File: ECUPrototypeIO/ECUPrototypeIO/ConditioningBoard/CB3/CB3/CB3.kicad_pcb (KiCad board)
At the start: 2 copper layers, 123.2 x 101.6 mm, 28 parts, among them J1 ECU Connector 1, J2 ECU Connector 2, J3 Relay Module Con2, J4 Vehicle Connector 1, J5 Relay Module Con1, Q1 MOSFET_A, SW1 MomentarySwitch, SW2 MomentarySwitch, T1 Screw_Terminal_01x04, U1 LM324

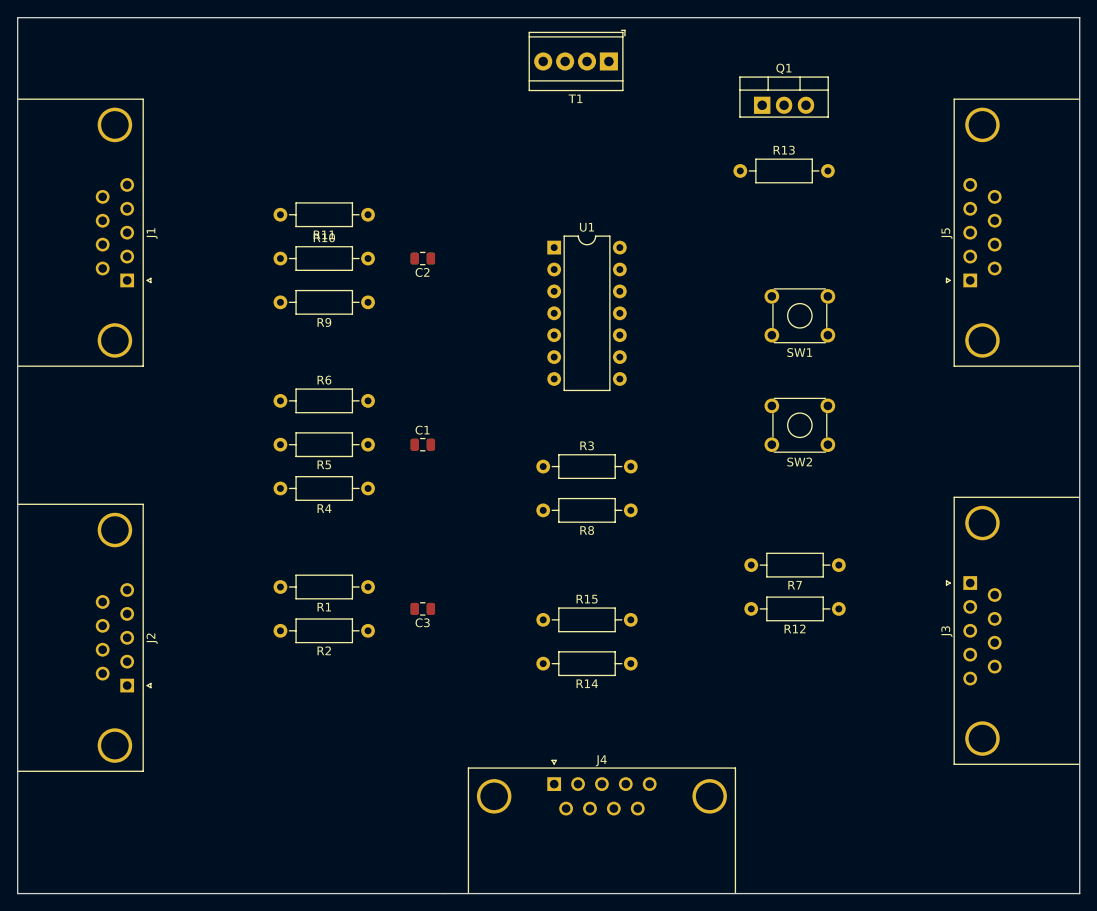
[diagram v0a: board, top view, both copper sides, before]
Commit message: latest files from jb laptop, unsure what changes exist
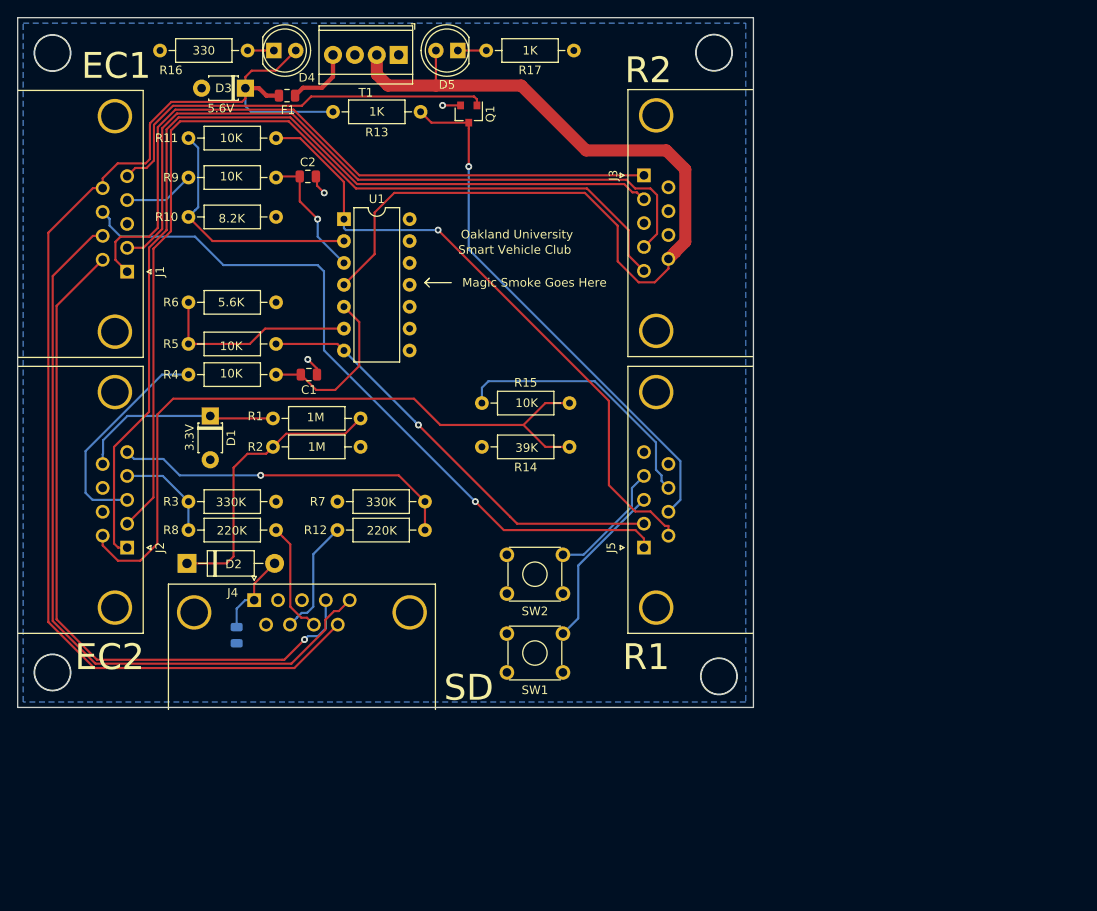
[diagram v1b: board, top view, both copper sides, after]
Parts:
- added D1: 3.3V, Diode_THT:D_T-1_P5.08mm_Horizontal, F.Cu at (96.0, 84.3)
- added D2: 1N4001, Diode_THT:D_DO-41_SOD81_P10.16mm_Horizontal, F.Cu at (93.3, 101.4)
- added D3: 5.6V, Diode_THT:D_T-1_P5.08mm_Horizontal, F.Cu at (100.1, 46.3)
- added D4: LD271, LED_THT:LED_D5.0mm_IRGrey, F.Cu at (103.4, 41.9)
- added D5: LD271, LED_THT:LED_D5.0mm_IRGrey, F.Cu at (124.7, 41.9)
- added F1: 1A Fuse, Fuse:Fuse_0805_2012Metric, F.Cu at (104.9, 47.1)
- added R16: 330, Resistor_THT:R_Axial_DIN0207_L6.3mm_D2.5mm_P10.16mm_Horizontal, F.Cu at (100.3, 41.9)
- added R17: 1K, Resistor_THT:R_Axial_DIN0207_L6.3mm_D2.5mm_P10.16mm_Horizontal, F.Cu at (128.0, 41.9)
- C3: moved to B.Cu
- Q1: value MOSFET_A -> 2N7002H; footprint Package_TO_SOT_THT:TO-220-3_Vertical -> Package_TO_SOT_SMD:SOT-23
- R12, R8: value 10K -> 220K
- R3, R7: value 20K -> 330K
- moved J3 60.6 mm to (146.3, 56.4)
- moved R12 58.9 mm to (110.7, 97.5), turned to 0 degrees
- moved SW1 49.7 mm to (136.9, 114.0)
- moved J5 48.9 mm to (146.3, 99.6)
- moved R7 48.6 mm to (120.9, 94.2)
- moved R3 41.3 mm to (93.5, 94.2)
- moved R8 41.2 mm to (103.6, 97.5)
- moved J4 40.8 mm to (101.1, 105.7)
- moved R13 37.7 mm to (120.4, 49.0), turned to 180 degrees
- moved SW2 35.3 mm to (136.9, 104.9)
- moved Q1 34.1 mm to (126.0, 49.3), turned to 270 degrees
- moved R15 26.1 mm to (127.5, 82.8)
- moved R14 26.1 mm to (137.7, 87.9)
- moved U1 24.6 mm to (111.5, 61.5)
- moved T1 24.4 mm to (117.9, 42.4)
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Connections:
- net +12V renamed 12V
- C1 pad 2: ReverseControl_Black -> GND
- C2 pad 2: ReverseControl_Black -> GND
- C3 pad 2: ReverseControl_Black -> GND
- J1 pad 0: (no net) -> GND
- J1 pad 3: ReverseControl_Black -> GND
- J1 pad 9: +5V -> 5V_Fused
- J2 pad 0: (no net) -> GND
- J3 pad 0: (no net) -> GND
- J3 pad 3: ReverseControl_Black -> GND
- J4 pad 0: (no net) -> GND
- J4 pad 2: ReverseControl_Black -> GND
- J4 pad 3: ReverseControl_Black -> GND
- J4 pad 6: ReverseControl_Black -> GND
- J4 pad 9: +5V -> 5V_Fused
- J5 pad 0: (no net) -> GND
- Q1 pad 2: RelayD_NO -> GND
- Q1 pad 3: ReverseControl_Black -> RelayD_NO
- R1 pad 1: MotorSpeed_Red -> Net-(D2-Pad1)
- R10 pad 2: ReverseControl_Black -> GND
- R13 pad 2: +5V -> 5V_Fused
- R14 pad 2: ReverseControl_Black -> GND
- R2 pad 1: ReverseControl_Black -> GND
- R2 pad 2: MotorSpeed_Red -> Net-(D2-Pad1)
- R3 pad 2: ReverseControl_Black -> GND
- R6 pad 2: ReverseControl_Black -> GND
- R7 pad 2: ReverseControl_Black -> GND
- SW1 pad 2: ReverseControl_Black -> GND
- SW2 pad 2: ReverseControl_Black -> GND
- T1 pad 1: ReverseControl_Black -> GND
- T1 pad 3: ReverseControl_Black -> GND
- T1 pad 4: +5V -> 5V
- U1 pad 1: (no net) -> RelayC_NO
- U1 pad 10: Net-(C2-Pad1) -> (no net)
- U1 pad 11: ReverseControl_Black -> GND
- U1 pad 2: (no net) -> Net-(R10-Pad1)
- U1 pad 3: (no net) -> Net-(C2-Pad1)
- U1 pad 8: RelayC_NO -> (no net)
- U1 pad 9: Net-(R10-Pad1) -> (no net)
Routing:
- net 5V_Fused: track 0.00 -> 141.8 mm
- net SteeringDirection: track 0.00 -> 112.2 mm
- net SteeringEnable: track 0.00 -> 111.9 mm
- net 12V: track 0.00 -> 111.3 mm
- net ReverseControl_Blue: track 0.00 -> 88.0 mm
- net Brake: track 0.00 -> 85.3 mm, vias 0 -> 1
- net SafetyLights2Enable: track 0.00 -> 85.3 mm
- net ReverseControl_Red: track 0.00 -> 81.9 mm, vias 0 -> 1
- net SafetyLights1Enable: track 0.00 -> 81.7 mm
- net ESTOP: track 0.00 -> 81.3 mm
- net RelayC_NO: track 0.00 -> 74.1 mm, vias 0 -> 1
- net RelayD_NO: track 0.00 -> 62.0 mm, vias 0 -> 1
- net SteeringDriverConnector1_Yellow: track 0.00 -> 51.3 mm, vias 0 -> 1
- net AccelerationEnable: track 0.00 -> 47.7 mm
- net SteeringEncoderB: track 0.00 -> 40.2 mm, vias 0 -> 1
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- added copper zone on B.Cu, net GND
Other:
- board size 123.2 x 101.6 mm -> 85.3 x 80 mm
- board text added: "10K"
- board text added: "1K"
- board text added: "1M"
- board text added: "220K"
- board text added: "3.3V"
- board text added: "330"
- board text added: "330K"
- board text added: "39K"
- board text added: "5.6K"
- board text added: "5.6V"
- board text added: "8.2K"
- board text added: "EC1"
- board text added: "EC2"
- board text added: "Magic Smoke Goes Here"
- board text added: "Oakland University"
- board text added: "R1"
- board text added: "R2"
- board text added: "SD"
- board text added: "Smart Vehicle Club"
